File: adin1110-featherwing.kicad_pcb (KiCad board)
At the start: 4 copper layers, 50.8 x 22.9 mm, 52 parts, among them J1 4039_Header_Male_Vert_16pin_0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, J2 4040_Header_Male_Vert_12pin_0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, J3 4060_TerminalBlock_NoScrew, SW1 4012_PushButton_NO_SMD, SW2 RST, T1 4057_Super_Tiny_Signal_Transf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, U1 4052_ADIN1110, U2 4058_TVS_2CH_Super_Speed, U3 LED0, U4 LED1, U5 LINK, Y1 4056_Crystal_25MHz

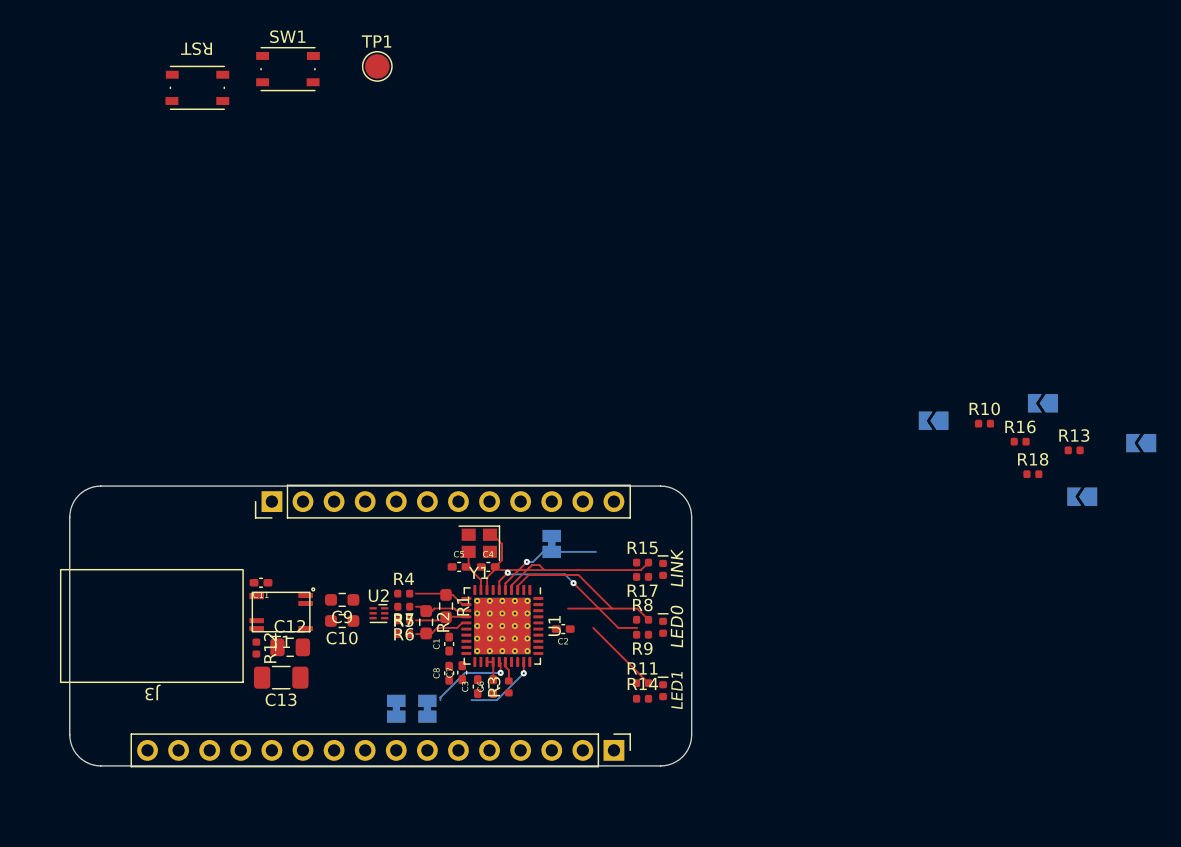
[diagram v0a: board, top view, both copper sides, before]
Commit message: ready to order
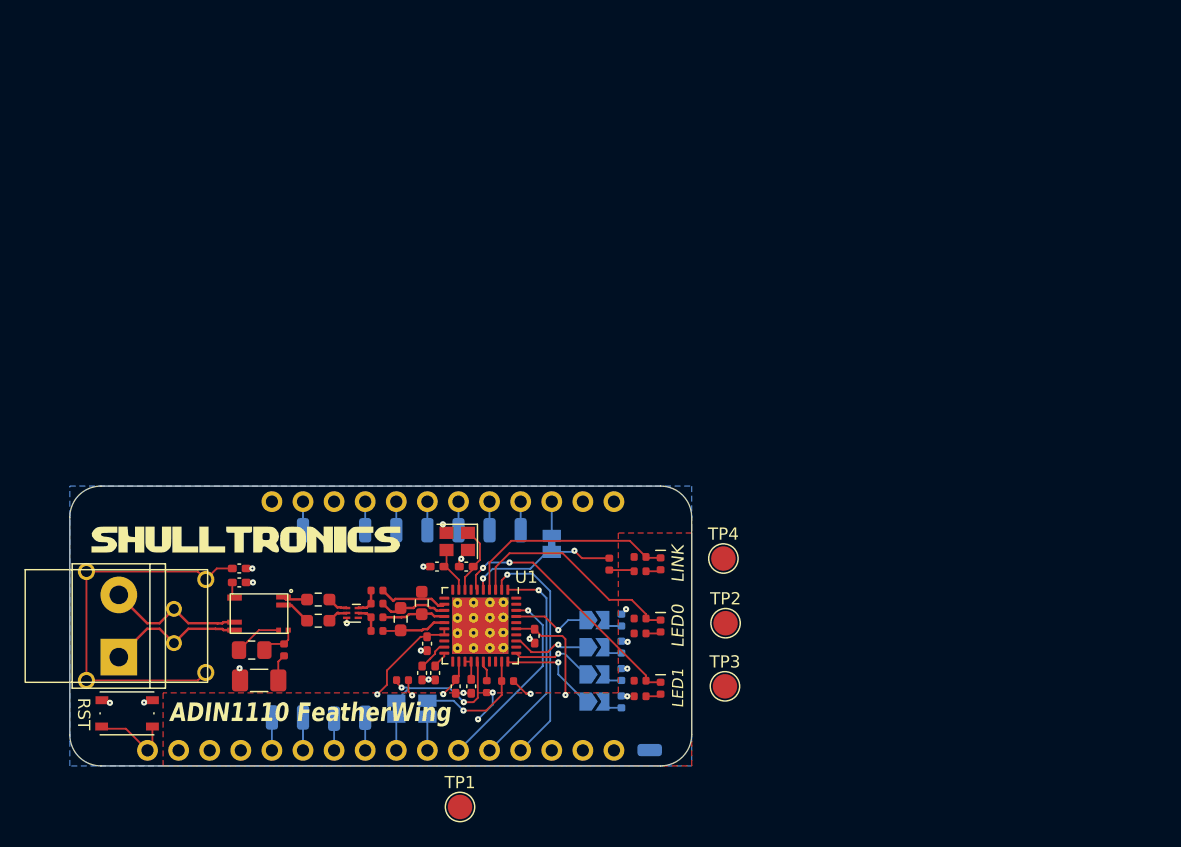
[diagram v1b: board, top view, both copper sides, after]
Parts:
- removed G***: LOGO, Shulltronics_Generics:LOGO-feather
- removed SW1: 4012_PushButton_NO_SMD, Shulltronics_ElectroMechanical:4012_PushButton_NO_SMD
- added ?: , , F.Cu at (151.1, 84.9)
- added C14: 4069_Capacitor_3.3n_50V_0402, Shulltronics_Generics:C_0402_HandSolder, F.Cu at (145.9, 88.0)
- added J4: ~, Shulltronics_Connectors:4067_SPE_IP20, F.Cu at (135.9, 92.7)
- added L1: Shulltronics_Logo, Shulltronics_Generics:Shulltronics_Logo, F.Cu at (145.7, 85.6)
- added R19: 4065_Resistor_SMD_1k5_0.10W_1%, Shulltronics_Generics:RES-0402, F.Cu at (159.3, 97.1)
- added R20: 4064_Resistor_SMD_4k7_0.10W_1%, Shulltronics_Generics:RES-0402, F.Cu at (167.8, 97.2)
- added R21: 4008_Resistor_SMD_10k_0.125W_1%, Shulltronics_Generics:RES-0402, F.Cu at (176.1, 87.7)
- added REF**: SolderWirePad_1x01_SMD_1x2mm, Connector_Wire:SolderWirePad_1x01_SMD_1x2mm, B.Cu at (166.4, 84.9)
- added REF**: SolderWirePad_1x01_SMD_1x2mm, Connector_Wire:SolderWirePad_1x01_SMD_1x2mm, B.Cu at (156.2, 84.9)
- added REF**: SolderWirePad_1x01_SMD_1x2mm, Connector_Wire:SolderWirePad_1x01_SMD_1x2mm, B.Cu at (158.8, 84.9)
- added REF**: SolderWirePad_1x01_SMD_1x2mm, Connector_Wire:SolderWirePad_1x01_SMD_1x2mm, B.Cu at (168.9, 84.9)
- added REF**: SolderWirePad_1x01_SMD_1x2mm, Connector_Wire:SolderWirePad_1x01_SMD_1x2mm, B.Cu at (179.5, 102.8)
- added REF**: SolderWirePad_1x01_SMD_1x2mm, Connector_Wire:SolderWirePad_1x01_SMD_1x2mm, B.Cu at (156.2, 100.2)
- added REF**: SolderWirePad_1x01_SMD_1x2mm, Connector_Wire:SolderWirePad_1x01_SMD_1x2mm, B.Cu at (161.3, 84.9)
- added REF**: SolderWirePad_1x01_SMD_1x2mm, Connector_Wire:SolderWirePad_1x01_SMD_1x2mm, B.Cu at (148.6, 100.2)
- added REF**: SolderWirePad_1x01_SMD_1x2mm, Connector_Wire:SolderWirePad_1x01_SMD_1x2mm, B.Cu at (153.7, 100.3)
- added REF**: SolderWirePad_1x01_SMD_1x2mm, Connector_Wire:SolderWirePad_1x01_SMD_1x2mm, B.Cu at (163.8, 84.9)
- added REF**: SolderWirePad_1x01_SMD_1x2mm, Connector_Wire:SolderWirePad_1x01_SMD_1x2mm, B.Cu at (151.1, 100.2)
- added TP2: LED0, Shulltronics_Generics:TestPoint_Pad_D2.0mm, F.Cu at (185.6, 92.5)
- added TP3: LED1, Shulltronics_Generics:TestPoint_Pad_D2.0mm, F.Cu at (185.6, 97.6)
- added TP4: LINK, Shulltronics_Generics:TestPoint_Pad_D2.0mm, F.Cu at (185.5, 87.2)
- J3: footprint Shulltronics_Connectors:4067_SPE_IP20 -> TerminalBlock:TerminalBlock_bornier-2_P5.08mm
- R10, R13, R16, R18: moved to B.Cu
- TP1: value TestPoint -> 1V1
- U1: footprint Package_DFN_QFN:QFN-40-1EP_6x6mm_P0.5mm_EP4.6x4.6mm_ThermalVias -> Shulltronics_Integrated_Circuits:4052_ADIN1110_40QFN
- moved TP1 60.9 mm to (164.0, 107.5)
- moved SW2 51.4 mm to (136.8, 99.9)
- moved JP5 47.0 mm to (174.9, 92.2), turned to 0 degrees
- moved JP7 43.2 mm to (174.9, 98.9), turned to 0 degrees
- moved JP6 41.7 mm to (174.9, 94.4), turned to 0 degrees
- moved R13 39.5 mm to (177.1, 92.2), turned to -90 degrees
- moved R18 38.4 mm to (177.1, 98.9), turned to -90 degrees
- moved R16 36.6 mm to (177.1, 94.4), turned to -90 degrees
- moved R10 36.0 mm to (177.1, 96.7), turned to -90 degrees
- moved JP4 34.6 mm to (174.9, 96.7), turned to 0 degrees
- moved J3 3.71 mm to (136.1, 95.2), turned to 90 degrees
- moved C12 3.15 mm to (146.9, 94.7), turned to 180 degrees
- moved C2 2.41 mm to (170.1, 93.5), turned to 90 degrees
- moved R12 2.27 mm to (149.6, 94.7)
- moved C7 2.21 mm to (161.9, 96.5)
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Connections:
- net /RXN renamed /RX-
- net /RXP renamed /RX+
- net /TXN renamed /TX-
- net /TXP renamed /TX+
- net Net-(C10-Pad1) renamed /Db-
- net Net-(C10-Pad2) renamed /Da-
- net Net-(C9-Pad1) renamed /Db+
- net Net-(C9-Pad2) renamed /Da+
- J1 pad 1: unconnected-(J1-Pad1) -> /USER
- J1 pad 10: unconnected-(J1-Pad10) -> /A2
- J1 pad 11: unconnected-(J1-Pad11) -> /A1
- J1 pad 12: unconnected-(J1-Pad12) -> /A0
- J1 pad 9: unconnected-(J1-Pad9) -> /A3
- J2 pad 4: unconnected-(J2-Pad4) -> /D13
- J2 pad 5: unconnected-(J2-Pad5) -> /D12
- J2 pad 6: unconnected-(J2-Pad6) -> /D11
- J2 pad 7: unconnected-(J2-Pad7) -> /D10
- J2 pad 8: unconnected-(J2-Pad8) -> /D9
- J2 pad 9: unconnected-(J2-Pad9) -> /D6
- JP2 pad 1: /~{RST} -> /~{RESET}
- R4 pad 1: Net-(R4-Pad1) -> /Dc+
- R5 pad 2: Net-(R4-Pad1) -> /Dc+
- R6 pad 2: Net-(R6-Pad2) -> /Dc-
- R7 pad 1: Net-(R6-Pad2) -> /Dc-
- SW2 pad 1: unconnected-(SW2-Pad1) -> /~{RST}
- SW2 pad 2: unconnected-(SW2-Pad2) -> GND
- TP1 pad 1: unconnected-(TP1-Pad1) -> /1V1
- U1 pad 5: /~{RST} -> /~{RESET}
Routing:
- net Net-(C14-Pad2): track 0.00 -> 31.5 mm
- net VCC: track 0.00 -> 28.8 mm, vias 0 -> 11
- net /MISO: track 0.00 -> 19.5 mm, vias 0 -> 1
- net /MOSI: track 0.00 -> 17.8 mm, vias 0 -> 1
- net /SCK: track 0.00 -> 15.7 mm, vias 0 -> 1
- net /~{RESET}: track 0.00 -> 12.4 mm, vias 0 -> 2
- net /D-: track 0.00 -> 11.4 mm
- net /D+: track 0.00 -> 11.4 mm
- net /MS_SEL: track 0.00 -> 8.27 mm, vias 0 -> 1
- net /~{TX2P4_EN}: track 0.00 -> 6.60 mm, vias 0 -> 1
- net /SPI_CFG1: track 0.00 -> 6.45 mm, vias 0 -> 1
- net /~{SWPD_EN}: track 0.00 -> 6.39 mm, vias 0 -> 1
- net /~{INT}: track 6.90 -> 12.1 mm, vias 1 -> 2
- net Net-(T1-OUT1B): track 0.00 -> 3.91 mm
- net /~{CS}: track 6.10 -> 9.66 mm
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- added copper zone on B.Cu, net GND
- added copper zone on F.Cu, net VCC
- removed copper zone on In1.Cu, net GND
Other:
- board text added: "ADIN1110 FeatherWing"
- board text added: "rev A"
